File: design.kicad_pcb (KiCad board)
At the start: 2 copper layers, 25 x 22.9 mm, 14 parts, among them J1 Conn_01x02, J2 Conn_01x02, J3 Conn_01x03, J4 Conn_01x03, U1 TPS61099YFFT

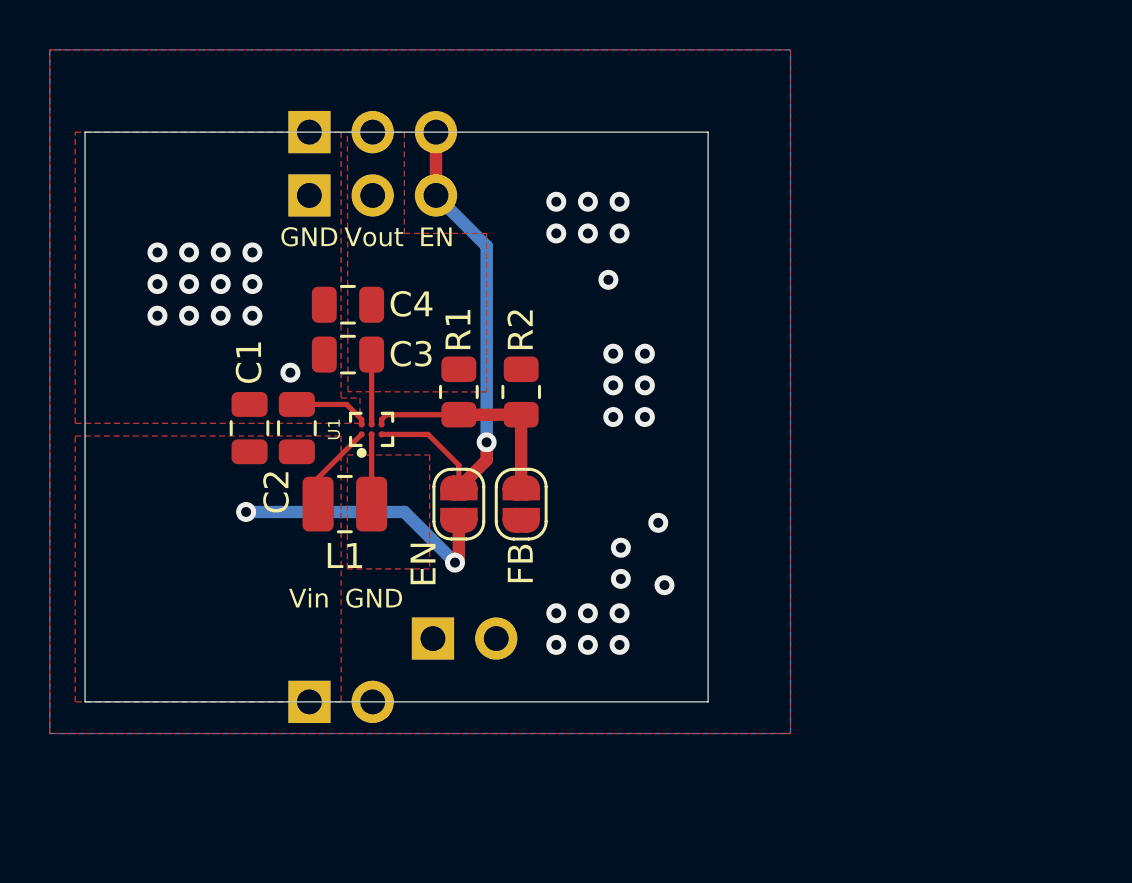
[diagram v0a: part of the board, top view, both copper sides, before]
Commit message: Update design.kicad_pcb
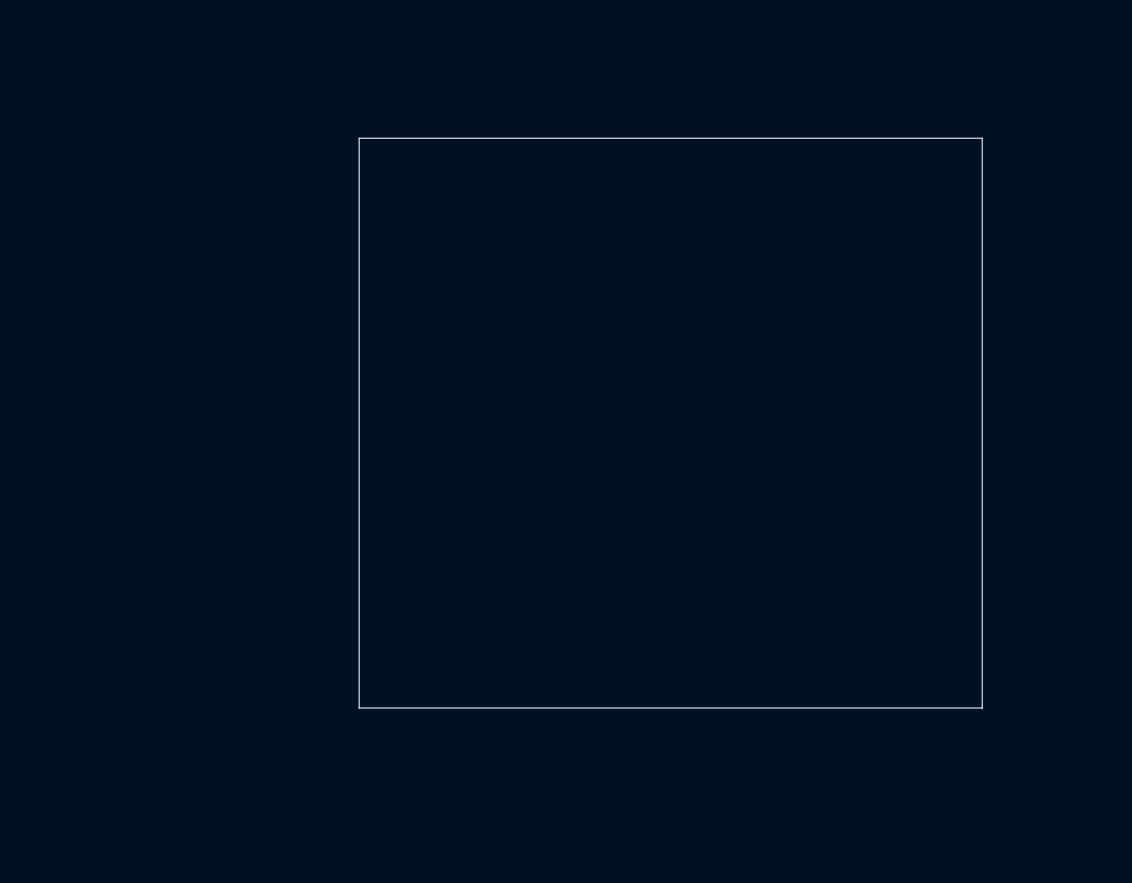
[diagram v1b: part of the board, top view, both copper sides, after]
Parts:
- removed C1, C2, C3, C4: C_Small, Capacitor_SMD:C_0805_2012Metric
- removed J1, J2: Conn_01x02, Connector_PinHeader_2.54mm:PinHeader_1x02_P2.54mm_Vertical
- removed J3, J4: Conn_01x03, Connector_PinHeader_2.54mm:PinHeader_1x03_P2.54mm_Vertical
- removed JP1, JP2: SolderJumper_2_Open, Jumper:SolderJumper-2_P1.3mm_Open_RoundedPad1.0x1.5mm
- removed L1: L_Small, Inductor_SMD:L_1008_2520Metric
- removed R1, R2: R_Small, Resistor_SMD:R_0805_2012Metric
- removed U1: TPS61099YFFT, Converter_DCDC_custom:BGA6N40P3X2_122X88X62N
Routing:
- net En: track 19.9 -> 0.00 mm, vias 1 -> 0
- net Vin: track 14.5 -> 0.00 mm, vias 2 -> 0
- net FB: track 8.82 -> 0.00 mm
- net GND: track 3.05 -> 0.00 mm, vias 36 -> 0
- net Vout: track 2.80 -> 0.00 mm
- net SW: track 2.80 -> 0.00 mm
- removed copper zone on B.Cu, net GND
- removed copper zone on F.Cu, net GND
- removed copper zone on F.Cu, net SW
- removed copper zone on F.Cu, net Vin
- removed copper zone on F.Cu, net Vout
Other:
- board text removed: "EN"
- board text removed: "GND"
- board text removed: "Vin"
- board text removed: "Vout"
